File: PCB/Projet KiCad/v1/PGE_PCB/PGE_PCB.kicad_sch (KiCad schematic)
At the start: 23 parts, among them J1 Conn_01x03_Pin, P1 USB_C_Plug_USB2.0, Q2 FDS4435BZ, U1 STM32L476RGTx, U2 LD1117S50TR_SOT223, U4 LD39050PU33R, Y1 ABS25-32.768KHZ-T

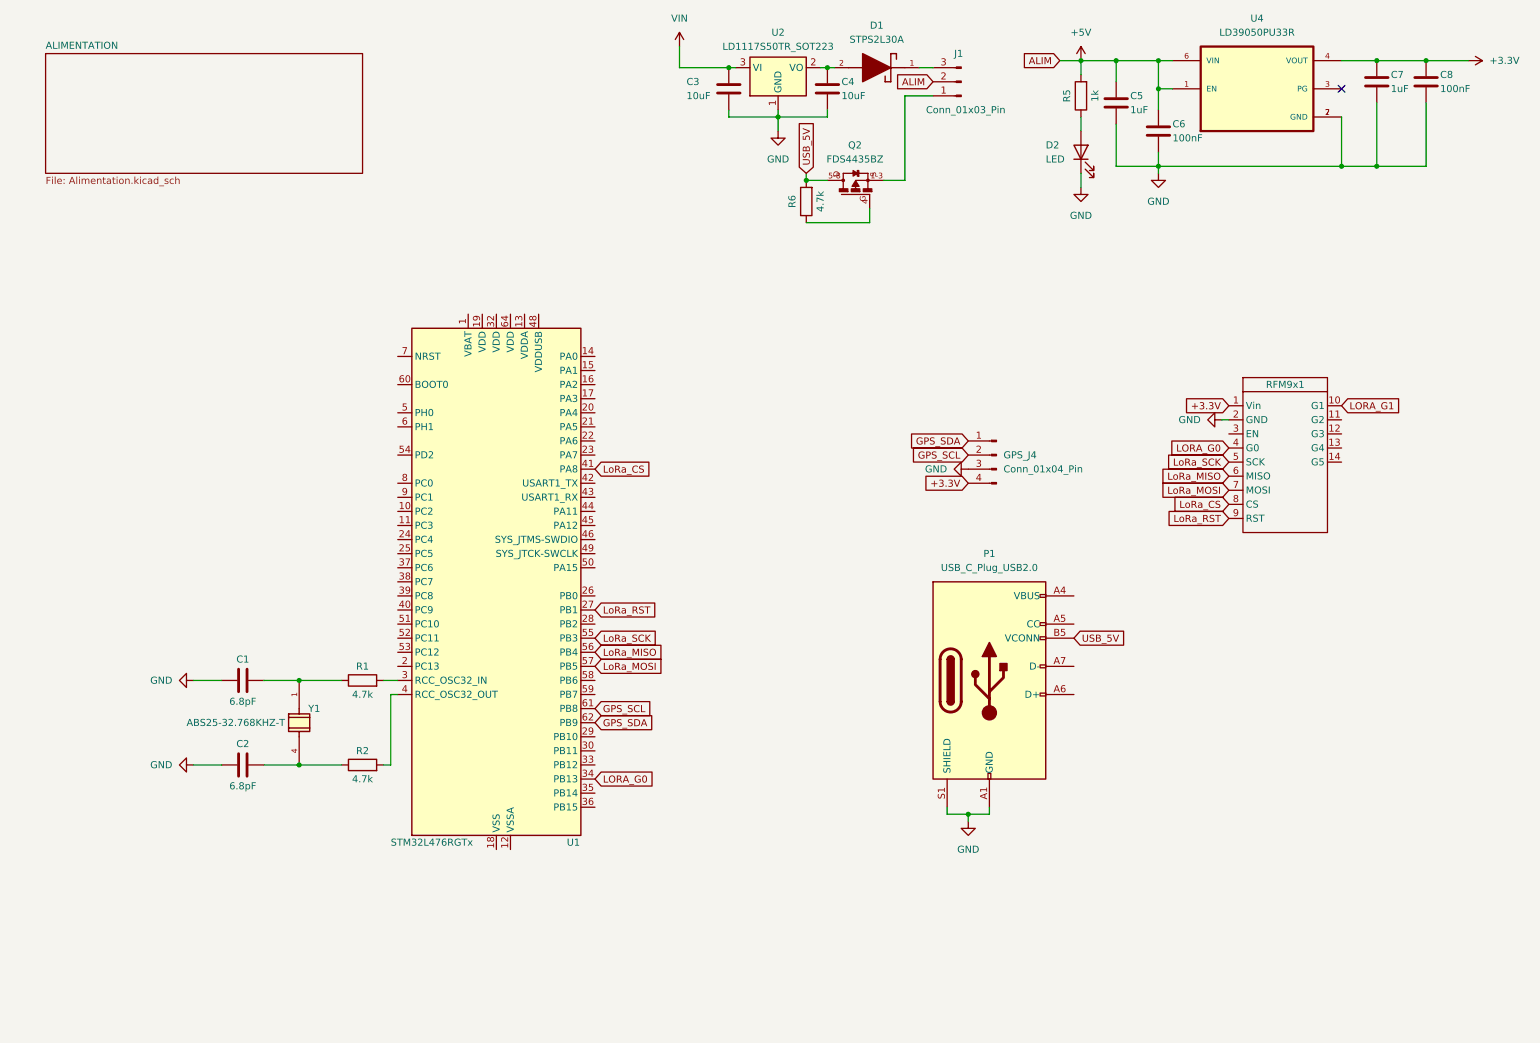
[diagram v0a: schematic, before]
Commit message: mise à jour Kicad
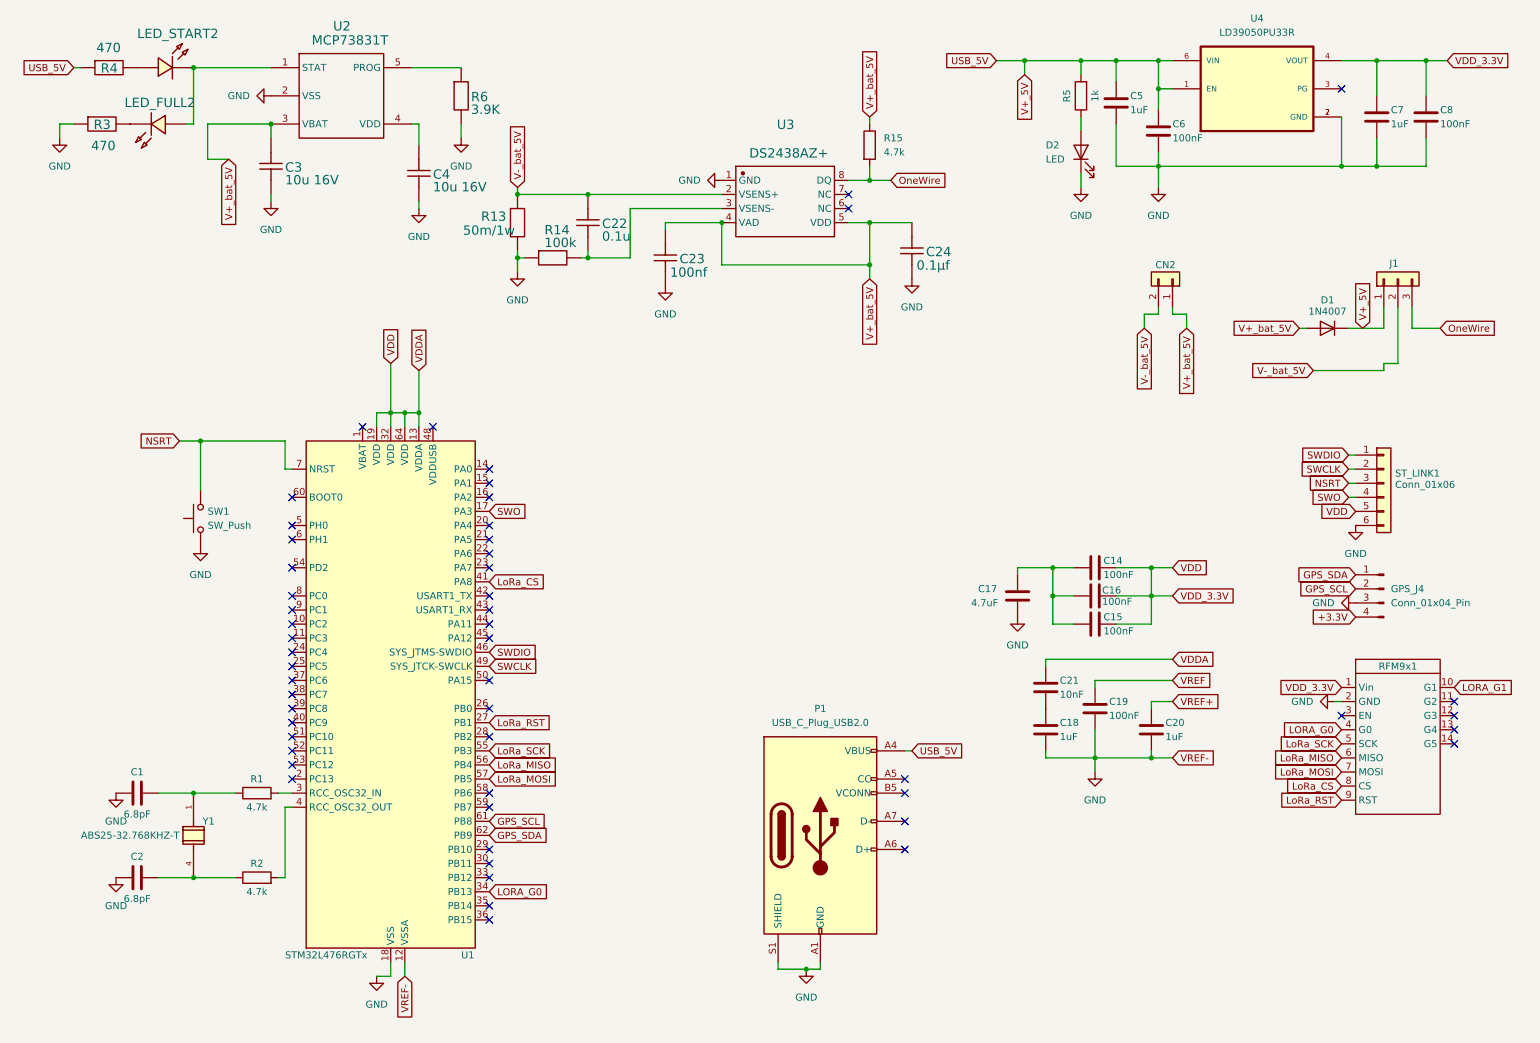
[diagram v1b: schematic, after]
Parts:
- removed C3, C4: 10uF, Capacitor_SMD:C_0603_1608Metric, symbol Device:C
- removed D1: STPS2L30A, STPS2L30A:DIOM5126X265N, symbol STPS2L30A:STPS2L30A
- removed J1: Conn_01x03_Pin, Connector_PinHeader_2.54mm:PinHeader_1x03_P2.54mm_Vertical, symbol Connector:Conn_01x03_Pin
- removed Q2: FDS4435BZ, FDS4435BZ:SO08-E3, symbol FDS4435BZ:FDS4435BZ
- removed R6: 4.7k, Resistor_SMD:R_0603_1608Metric, symbol Device:R
- removed U2: LD1117S50TR_SOT223, Package_TO_SOT_SMD:SOT-223-3_TabPin2, symbol Regulator_Linear:LD1117S50TR_SOT223
- added C14, C15, C16, C19: 100nF, Capacitor_SMD:C_0805_2012Metric, symbol Device:C
- added C17: 4.7uF, Capacitor_SMD:C_0805_2012Metric, symbol Device:C
- added C18, C20: 1uF, Capacitor_SMD:C_0805_2012Metric, symbol Device:C
- added C21: 10nF, Capacitor_SMD:C_0805_2012Metric, symbol Device:C
- added C22: 0.1u, Capacitor_SMD:C_0805_2012Metric, symbol C_0805_US_2
- added C23: 100nf, Capacitor_SMD:C_0805_2012Metric, symbol C_0805_US_3
- added C24: 0.1µf, Capacitor_SMD:C_0805_2012Metric, symbol C_0805_US_4
- added C3: 10u 16V, Capacitor_SMD:C_0805_2012Metric, symbol C_0805_US_1
- added C4: 10u 16V, Capacitor_SMD:C_0805_2012Metric, symbol C_0805_US
- added CN2: Conn_01x02, TerminalBlock_MetzConnect:TerminalBlock_MetzConnect_Type011_RT05502HBWC_1x02_P5.00mm_Horizontal, symbol Connector_Generic:Conn_01x02
- added D1: 1N4007, Diode_SMD:D_SMA, symbol Diode:1N4007
- added J1: Conn_01x03, Connector_PinHeader_2.54mm:PinHeader_1x03_P2.54mm_Vertical, symbol Connector_Generic:Conn_01x03
- added LED_FULL2: LED-0805_G, LED_SMD:LED_0805_2012Metric, symbol LED-0805_G
- added LED_START2: LED-0603_B, LED_SMD:LED_0805_2012Metric, symbol LED-0603_B
- added R13: 50m/1w, Resistor_SMD:R_0805_2012Metric, symbol R_0805_EU_3
- added R14: 100k, Resistor_SMD:R_0805_2012Metric, symbol R_0805_EU_4
- added R15: 4.7k, Resistor_SMD:R_0805_2012Metric, symbol Device:R
- added R3: 470, Resistor_SMD:R_0805_2012Metric, symbol R_0805_EU_2
- added R4: 470, Resistor_SMD:R_0805_2012Metric, symbol R_0805_EU_1
- added R6: 3.9K, Resistor_SMD:R_0805_2012Metric, symbol R_0805_EU
- added ST_LINK1: Conn_01x06, Connector_JST:JST_EH_B6B-EH-A_1x06_P2.50mm_Vertical, symbol Connector_Generic:Conn_01x06
- added SW1: SW_Push, Button_Switch_SMD:SW_SPST_CK_KMS2xxGP, symbol Switch:SW_Push
- added U2: MCP73831T, Package_TO_SOT_SMD:SOT-23-5, symbol MCP73831T-2ATI/OT
- added U3: DS2438AZ+, Package_SO:SOIC-8_3.9x4.9mm_P1.27mm, symbol DS2438AZ+
- C1, C2, C5, C6, C7, C8: footprint Capacitor_SMD:C_0603_1608Metric -> Capacitor_SMD:C_0805_2012Metric
- GPS_J4: footprint Connector_PinHeader_1.00mm:PinHeader_1x04_P1.00mm_Vertical -> Connector_PinHeader_2.54mm:PinHeader_1x04_P2.54mm_Vertical
- R1, R2: footprint Capacitor_SMD:C_0201_0603Metric -> Resistor_SMD:R_0805_2012Metric
- R5: footprint Resistor_SMD:R_0603_1608Metric -> Resistor_SMD:R_0805_2012Metric
- U4: footprint LD39050PU33R:SON95P300X300X100-7N -> Package_DFN_QFN:DFN-6-1EP_3x3mm_P0.95mm_EP1.7x2.6mm
- Y1: footprint ABS25-32.768KHZ-T:XTAL_ABS25-32.768KHZ-6-1-T -> Oscillator:XTAL_ABS25-32.768KHZ-6-1-T
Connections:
- net +5V is gone; now on net USB_5V: C5.1, C6.1, R5.2, U4.1 (EN), U4.6 (VIN)
- net +3.3V: no longer C7.1, C8.1, RFM9x1.1 (Vin), U4.4 (VOUT)
- net GND: now also U1.12 (VSSA), U1.18 (VSS), U1.31 (VSS), U1.47 (VSS), U1.63 (VSS), C17.2, C18.2, C19.2, C20.2, C23.1, C24.1, C3.1, C4.1, R13.1, R14.2, R3.2, R6.1, ST_LINK1.6 (Pin_6), SW1.1, U2.2 (VSS), U3.1 (GND)
- net USB_5V: now also P1.A4 (VBUS), P1.A9 (VBUS), P1.B4 (VBUS), P1.B9 (VBUS), D1.1 (K), J1.1 (Pin_1), R4.2; no longer P1.B5 (VCONN)
- net VDD: now reaches U1.13 (VDDA)
- net VDD: now also C7.1, C8.1, RFM9x1.1 (Vin), U1.19 (VDD), U1.32 (VDD), U1.64 (VDD), U4.4 (VOUT), C14.1, C15.1, C16.1, C21.1, ST_LINK1.5 (Pin_5)
- net SWO: now reaches U1.17 (PA3)
- net SWO: now also ST_LINK1.4 (Pin_4)
- net SWDIO: now reaches U1.46 (PA13)
- net SWDIO: now also ST_LINK1.1 (Pin_1)
- net SWCLK: now reaches U1.49 (PA14)
- net SWCLK: now also ST_LINK1.2 (Pin_2)
- net NSRT: now reaches U1.7 (NRST)
- net NSRT: now also ST_LINK1.3 (Pin_3), SW1.2
- new net: C22.1, R14.1, U3.3 (VSENS-)
- new net: LED_START2.1, R4.1
- new net: LED_FULL2.1, LED_START2.2, U2.1 (STAT)
- new net: C14.2, C15.2, C16.2, C17.1
- new net: LED_FULL2.2, R3.1
- new net: C4.2, U2.4 (VDD)
- new net: R6.2, U2.5 (PROG)
- new net: C18.1, C21.2
- new net OneWire: J1.3 (Pin_3), R15.2, U3.8 (DQ)
- new net V+_bat_5V: C23.2, C24.2, C3.2, CN2.1 (Pin_1), D1.2 (A), R15.1, U2.3 (VBAT), U3.4 (VAD), U3.5 (VDD)
- new net V-_bat_5V: C22.2, CN2.2 (Pin_2), J1.2 (Pin_2), R13.2, U3.2 (VSENS+)
- new net VREF: C19.1
- new net VREF+: C20.1
- no-connect marks 1 -> 53
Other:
- removed sheet ALIMENTATION
- moved on the sheet: C1, C2, C7, C8, GPS_J4, P1, R1, R2, RFM9x1, U1, Y1

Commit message: fin routage prototype_V1
Pour avis Kristen
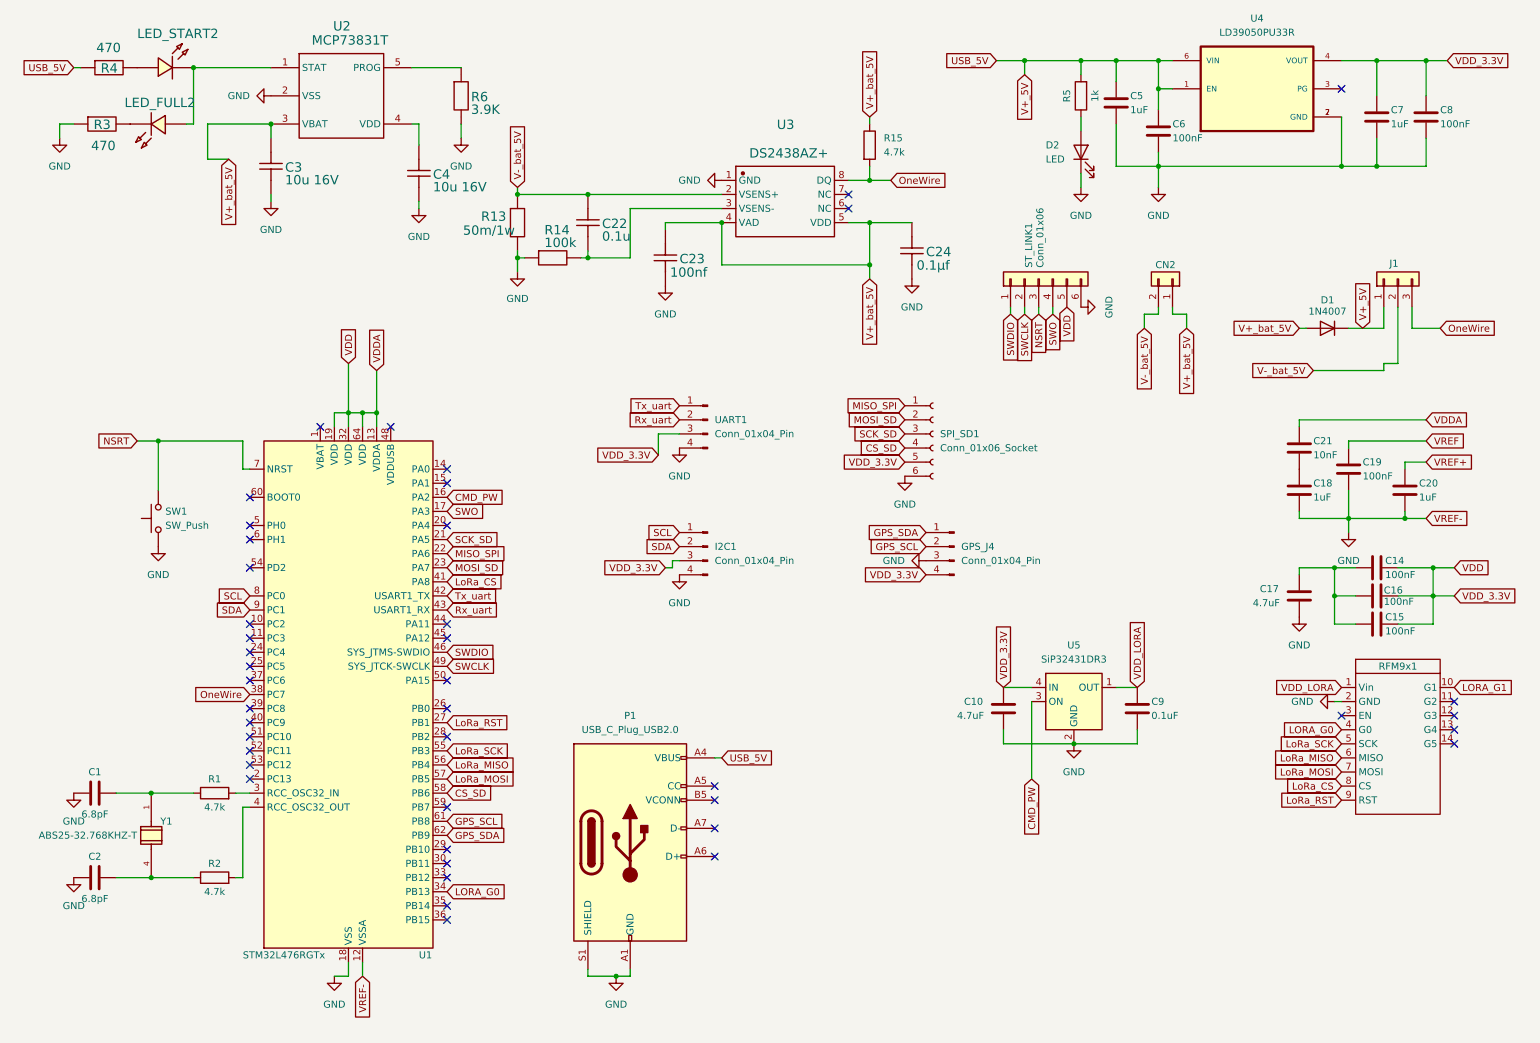
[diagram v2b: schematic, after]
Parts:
- added C10: 4.7uF, Capacitor_SMD:C_0805_2012Metric, symbol Device:C
- added C9: 0.1uF, Capacitor_SMD:C_0805_2012Metric, symbol Device:C
- added I2C1, UART1: Conn_01x04_Pin, Connector_PinHeader_2.54mm:PinHeader_1x04_P2.54mm_Vertical, symbol Connector:Conn_01x04_Pin
- added SPI_SD1: Conn_01x06_Socket, Connector_PinHeader_2.54mm:PinHeader_1x06_P2.54mm_Vertical, symbol Connector:Conn_01x06_Socket
- added U5: SiP32431DR3, Package_TO_SOT_SMD:SOT-363_SC-70-6, symbol Power_Management:SiP32431DR3
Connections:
- net +3.3V is gone; now on net VDD: GPS_J4.4 (Pin_4)
- net GND: now also C10.2, C9.2, I2C1.4 (Pin_4), SPI_SD1.6 (Pin_6), U5.2 (GND), U5.5 (GND), UART1.4 (Pin_4)
- net OneWire: now also U1.38 (PC7)
- net VDD: now also C10.1, I2C1.3 (Pin_3), SPI_SD1.5 (Pin_5), U5.4 (IN), UART1.3 (Pin_3); no longer RFM9x1.1 (Vin)
- net CMD_PW: now reaches U1.16 (PA2)
- net CMD_PW: now also U5.3 (ON)
- net SCK_SD: now reaches U1.21 (PA5)
- net SCK_SD: now also SPI_SD1.3 (Pin_3)
- net MISO_SPI: now reaches U1.22 (PA6)
- net MISO_SPI: now also SPI_SD1.1 (Pin_1)
- net MOSI_SD: now reaches U1.23 (PA7)
- net MOSI_SD: now also SPI_SD1.2 (Pin_2)
- net Tx_uart: now reaches U1.42 (PA9)
- net Tx_uart: now also UART1.1 (Pin_1)
- net Rx_uart: now reaches U1.43 (PA10)
- net Rx_uart: now also UART1.2 (Pin_2)
- net CS_SD: now reaches U1.58 (PB6)
- net CS_SD: now also SPI_SD1.4 (Pin_4)
- net SCL: now reaches U1.8 (PC0)
- net SCL: now also I2C1.1 (Pin_1)
- net SDA: now reaches U1.9 (PC1)
- net SDA: now also I2C1.2 (Pin_2)
- new net VDD_LORA: C9.1, RFM9x1.1 (Vin), U5.1 (OUT)
- no-connect marks 53 -> 43
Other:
- moved on the sheet: C1, C14, C15, C16, C17, C18, C19, C2, C20, C21, GPS_J4, P1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
